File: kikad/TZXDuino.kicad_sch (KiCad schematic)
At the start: 22 parts, among them J1 SPECCY, J2 SPEAKER, J3 POWER IN, J4 SD_Card, SW1 CHERRY MX, SW2 CHERRY MX, SW3 CHERRY MX, SW4 CHERRY MX, U1 ARDUINO NANO, U2 LCD 1602

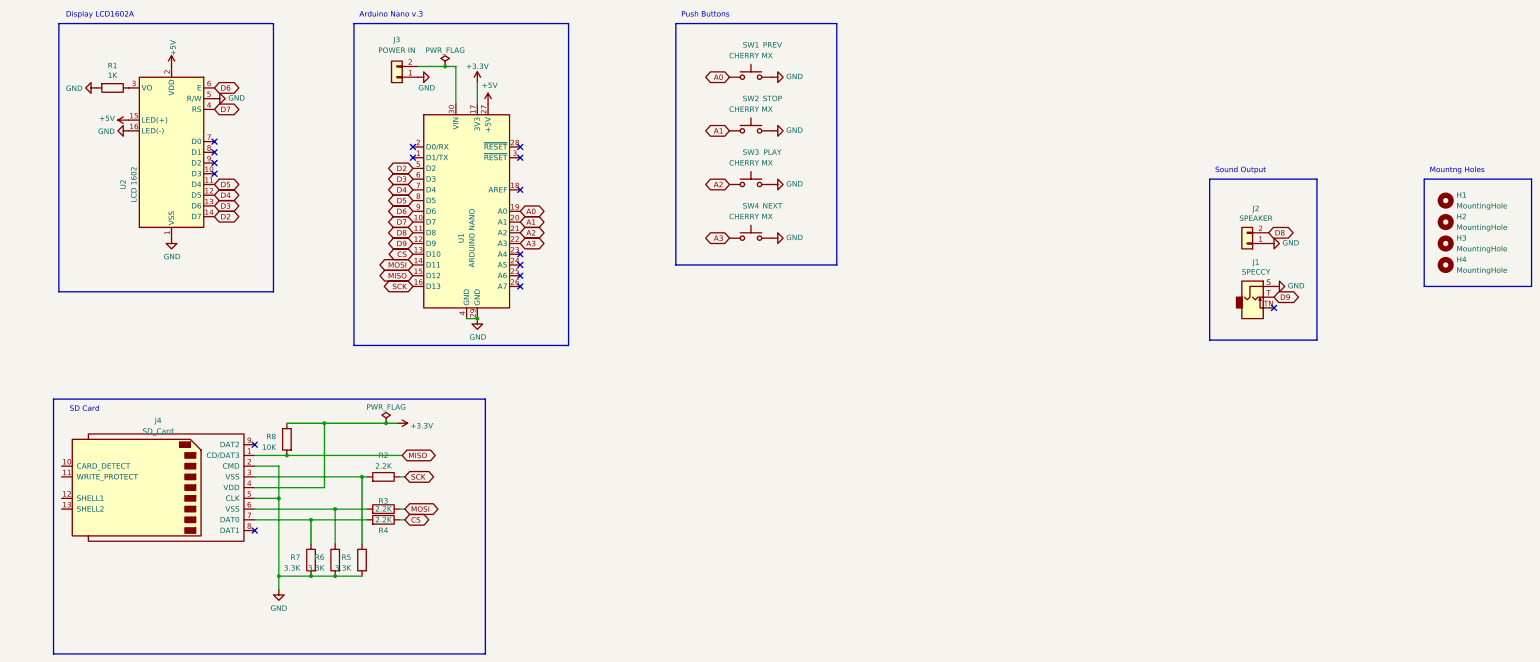
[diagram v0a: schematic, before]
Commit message: Update
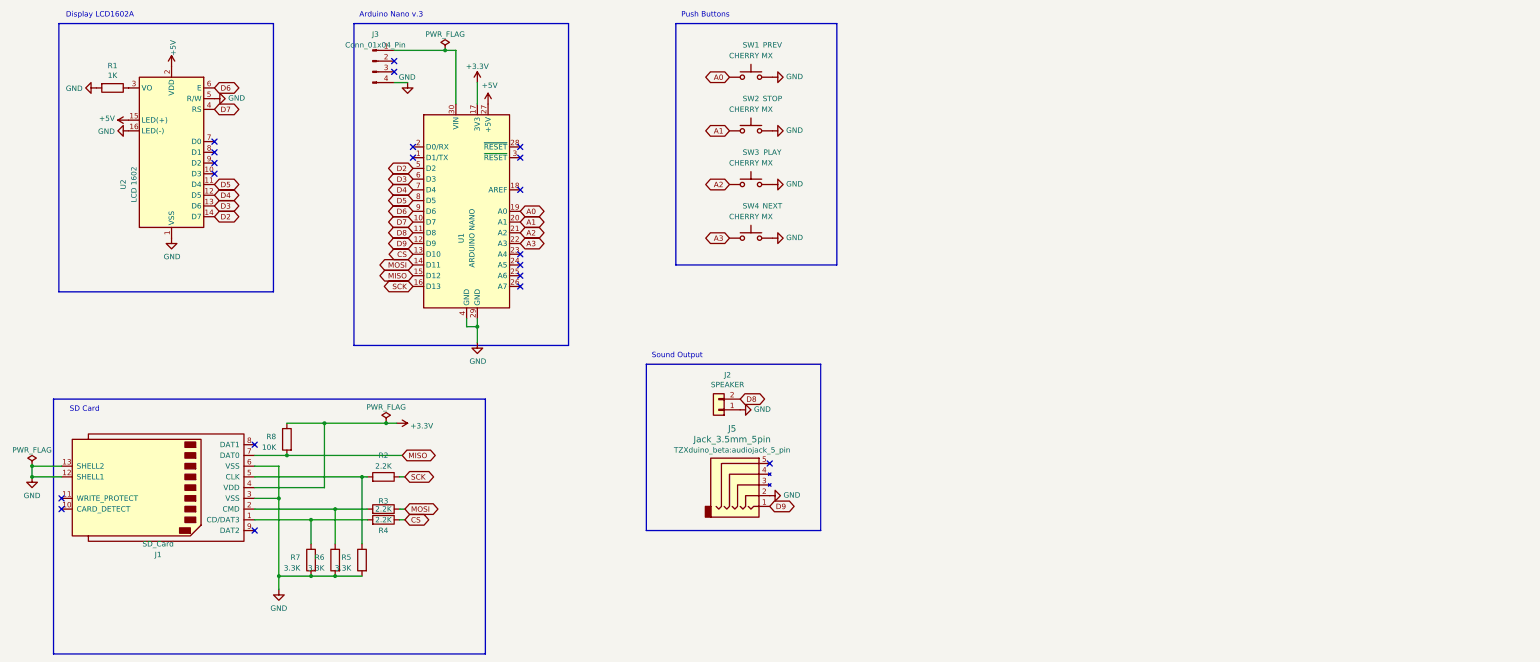
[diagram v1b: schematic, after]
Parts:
- removed H1, H2, H3, H4: MountingHole, MountingHole:MountingHole_3mm_Pad, symbol tzxduino_pre:MountingHole
- removed J1: SPECCY, TZXDuino:PJ-316, symbol tzxduino_pre:AudioJack2_SwitchT-Connector
- removed J3: POWER IN, TZXDuino:PinHeader_1x02_P2.54mm_Horizontal, symbol tzxduino_pre:Conn_01x02
- removed J4: SD_Card, TZXduino_beta:SDCARD_4UCONN, symbol tzxduino_pre:SD_Card
- added J1: SD_Card, TZXduino_beta:SDCARD_4UCONN, symbol tzxduino_pre:SD_Card
- added J3: Conn_01x04_Pin, TZXduino_beta:USB-C Power board, symbol Connector:Conn_01x04_Pin
- added J5: Jack_3.5mm_5pin, TZXduino_beta:audiojack_5_pin, symbol tzxduino_pre:AudioJack_5_pin
- J2: footprint Connector_PinHeader_2.54mm:PinHeader_1x02_P2.54mm_Vertical -> TZXduino_beta:Speaker
- R1: footprint Resistor_THT:R_Axial_DIN0204_L3.6mm_D1.6mm_P7.62mm_Horizontal -> R_Axial_DIN0207_L6.3mm_D2.5mm_P10.16mm_Horizontal
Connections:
- net +3.3V: now also J1.4 (VDD)
- net D9: now also J5.1
- net GND: now also J1.12 (SHELL1), J1.13 (SHELL2), J1.3 (VSS), J1.6 (VSS), J3.4 (Pin_4), J5.2
- net MISO: now also J1.7 (DAT0)
- net at U1.30 (VIN): now also J3.1 (Pin_1)
- net at R2.2, R5.1: now also J1.5 (CLK)
- net at R3.2, R6.1: now also J1.2 (CMD)
- net at R4.2, R7.1: now also J1.1 (CD/DAT3)
- no-connect marks 16 -> 20
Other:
- note removed: "Mountng Holes"
- moved on the sheet: J2
